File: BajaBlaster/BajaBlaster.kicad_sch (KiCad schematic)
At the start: 0 parts

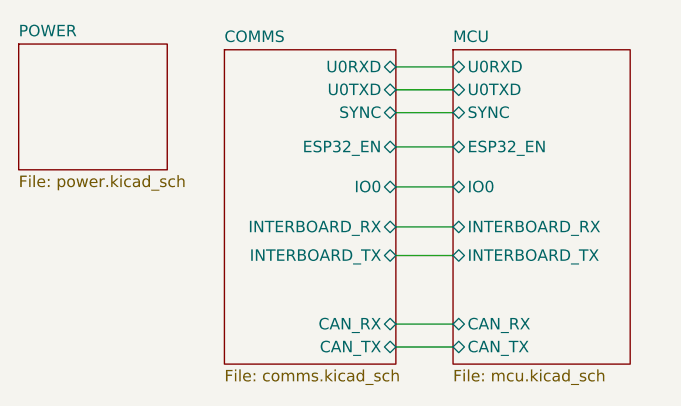
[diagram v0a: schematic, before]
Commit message: sendoff
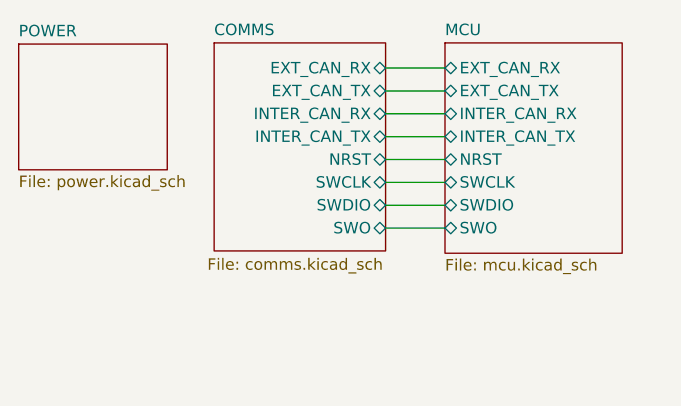
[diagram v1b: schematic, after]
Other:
- sheet COMMS ports: added EXT_CAN_RX, EXT_CAN_TX, INTER_CAN_RX, INTER_CAN_TX, NRST, SWCLK, SWDIO, SWO; removed CAN_RX, CAN_TX, ESP32_EN, INTERBOARD_RX, INTERBOARD_TX, IO0, SYNC, U0RXD, U0TXD
- sheet MCU ports: added EXT_CAN_RX, EXT_CAN_TX, INTER_CAN_RX, INTER_CAN_TX, NRST, SWCLK, SWDIO, SWO; removed CAN_RX, CAN_TX, ESP32_EN, INTERBOARD_RX, INTERBOARD_TX, IO0, SYNC, U0RXD, U0TXD
